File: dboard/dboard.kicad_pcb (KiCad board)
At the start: 2 copper layers, 49 x 11 mm, 10 parts, among them J1 Conn_01x04, U1 SRV05-4

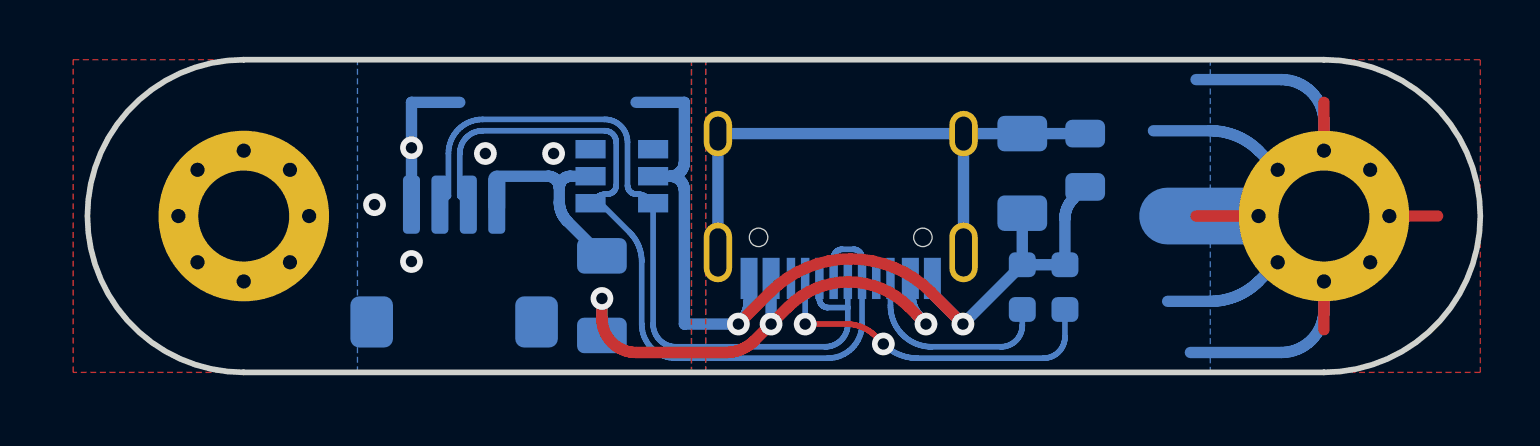
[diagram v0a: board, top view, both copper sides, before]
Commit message: a bunch of new dboards
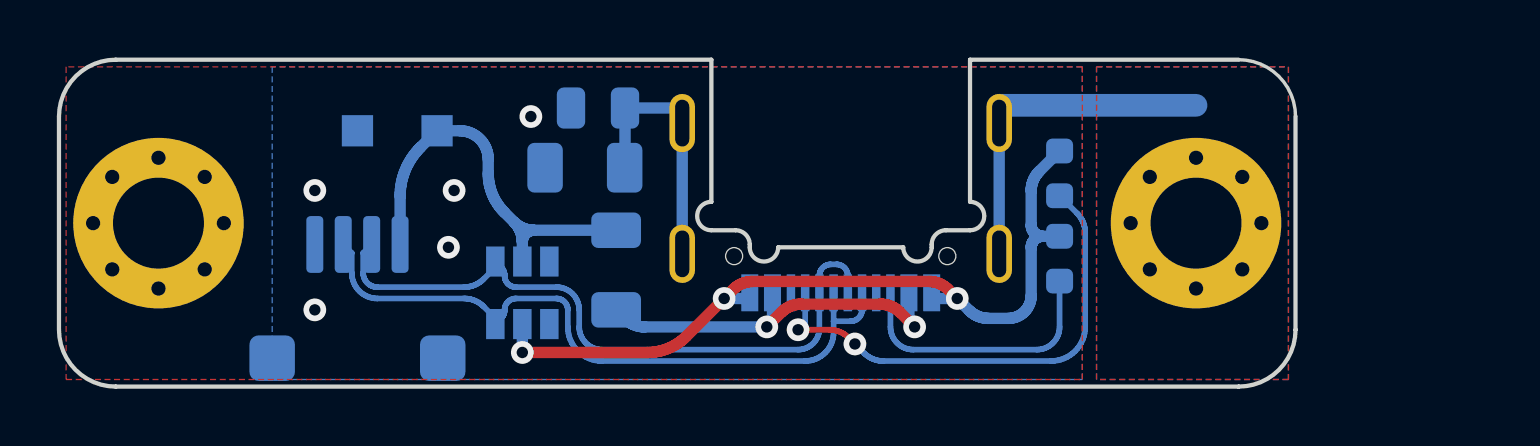
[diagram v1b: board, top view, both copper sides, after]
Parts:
- added D1: D_TVS, Diode_SMD:D_SOD-123F, B.Cu at (-15.6, 2.50)
- H2: moved to B.Cu
- J1: value Conn_01x04 -> JST_SH_SM04B-SRSS-TB_1x04
- USB1: value HRO-TYPE-C-31-M-12 -> HRO-TYPE-C-31-M-14; footprint Type-C:HRO-TYPE-C-31-M-12-Assembly -> Type-C:HRO-TYPE-C-31-M-14
- moved C1 17.2 mm to (-8.54, 1.70), turned to 180 degrees
- moved R3 15.4 mm to (-9.00, 3.80), turned to 180 degrees
- moved U1 5.39 mm to (-11.2, 8.20), turned to 90 degrees
- moved J1 5.21 mm to (-17.0, 11.3)
- moved H2 4.51 mm to (12.5, 5.75), turned to 180 degrees
- moved R1 4.00 mm to (7.70, 4.00)
- moved H1 3.01 mm to (-24.0, 5.75), turned to 180 degrees
- moved R2 1.65 mm to (7.70, 7.00)
- moved F1 1.03 mm to (-7.90, 7.40)
- turned USB1 to 180 degrees
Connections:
- J1 pad 2: D+ -> D-
- J1 pad 3: D- -> D+
- U1 pad 3: D- -> D+
- U1 pad 4: D+ -> D-
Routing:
- net SHIELD: track 74.6 -> 20.3 mm
- net GND: track 40.3 -> 29.1 mm, vias 7 -> 8
- net +5V: track 7.74 -> 15.1 mm
- net Net-(R1-Pad2): track 12.5 -> 17.5 mm
- net VBUS: track 18.8 -> 13.9 mm, vias 3 -> 2
- net D+: track 29.5 -> 24.9 mm
- net D-: track 27.6 -> 24.3 mm
- net Net-(R2-Pad2): track 7.41 -> 9.67 mm
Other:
- board size 49 x 11 mm -> 43.5 x 11.5 mm
- net class Default: clearance 0.2 -> 0.18
- net class Power: clearance 0.2 -> 0.18
- rule trace_clearance: 0.2 -> 0.18
